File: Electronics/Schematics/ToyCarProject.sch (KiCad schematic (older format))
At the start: 25 parts

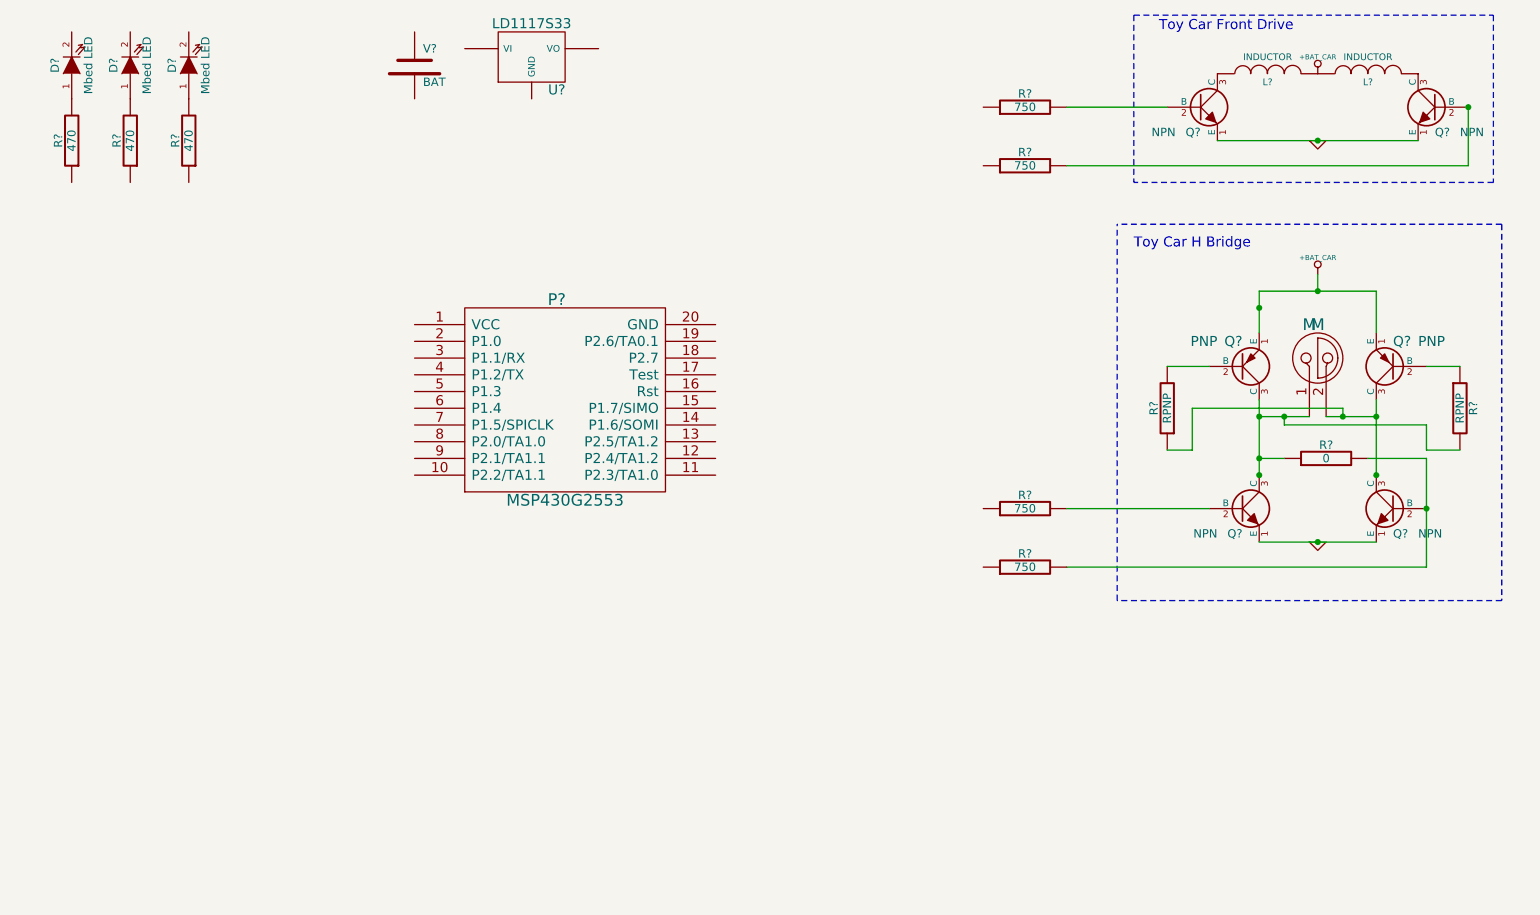
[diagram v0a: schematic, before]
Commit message: Project Schematic Update
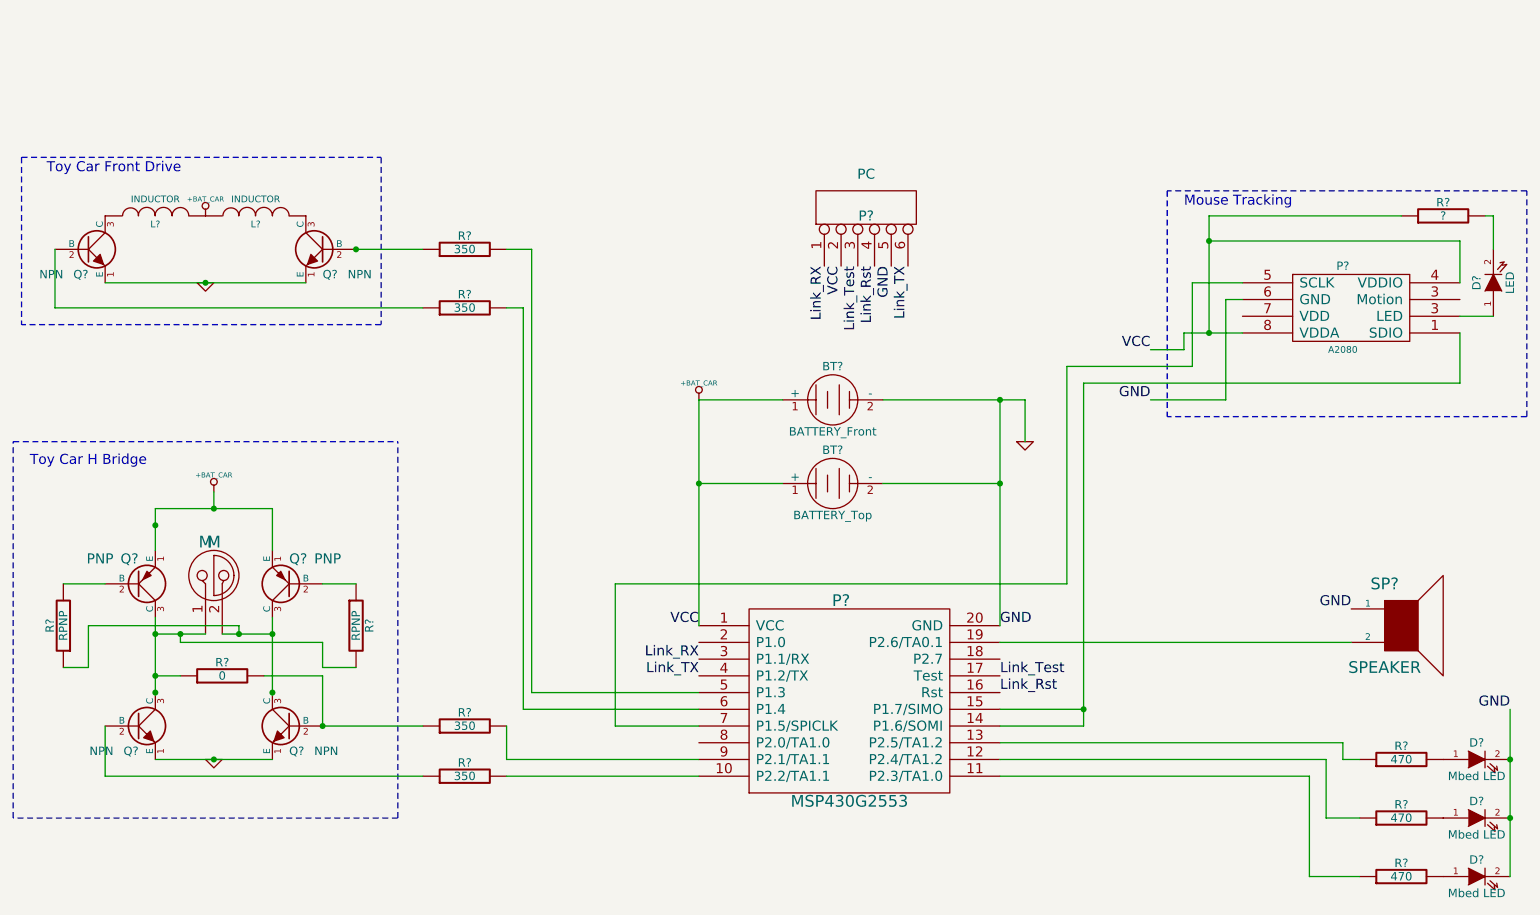
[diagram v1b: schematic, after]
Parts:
- removed U?: LD1117S33, symbol LM7805
- removed V?: BAT, symbol BAT
- added BT?: BATTERY_Front, symbol BATTERY
- added BT?: BATTERY_Top, symbol BATTERY
- added D?: LED, symbol LED
- added P?: A2080, symbol A2080
- added P?: PC, symbol CONN_6
- added R?: ?, symbol R
- added SP?: SPEAKER, symbol SPEAKER
- R? (x4): value 750 -> 350
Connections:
- net +BAT_CAR: now also P?.1 (VCC), BT?.1 (+), BT?.1 (+), P?.2, P?.4 (VDDIO), P?.8 (VDDA), R?.1
- net GND: now also D?.2 (K), D?.2 (K), D?.2 (K), P?.20 (GND), BT?.2 (-), BT?.2 (-), P?.5, P?.6 (GND), SP?.1
- net at Q?.2 (B): now also R?.1; no longer R?.2
- net at Q?.2 (B), R?.2: now also R?.1; no longer R?.2
- net at R?.1: now also Q?.2 (B) (x2)
- net at R?.2: now also P?.5 (P1.3); no longer Q?.2 (B)
- net at R?.2: now also P?.6 (P1.4); no longer Q?.2 (B)
- net at R?.1: now also P?.13 (P2.5/TA1.2)
- net at R?.1: now also P?.12 (P2.4/TA1.2)
- net at R?.1: now also P?.11 (P2.3/TA1.0)
- net at P?.10 (P2.2/TA1.1): now also R?.2
- net at P?.14 (P1.6/SOMI): now also P?.15 (P1.7/SIMO), P?.1 (SDIO)
- net Link_Rst: now reaches P?.16 (Rst)
- net Link_Rst: now also P?.4
- net Link_Test: now reaches P?.17 (Test)
- net Link_Test: now also P?.3
- net at P?.19 (P2.6/TA0.1): now also SP?.2
- net Link_RX: now reaches P?.3 (P1.1/RX)
- net Link_RX: now also P?.1
- net Link_TX: now reaches P?.4 (P1.2/TX)
- net Link_TX: now also P?.6
- net at P?.7 (P1.5/SPICLK): now also P?.5 (SCLK)
- net at P?.9 (P2.1/TA1.1): now also R?.2
- new net: D?.1 (A), P?.3 (Motion)
- new net: D?.2 (K), R?.2
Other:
- note added: "Mouse Tracking"
- moved on the sheet: D?, L?, M, P?, Q?, R?
